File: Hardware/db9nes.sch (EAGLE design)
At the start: 3 parts

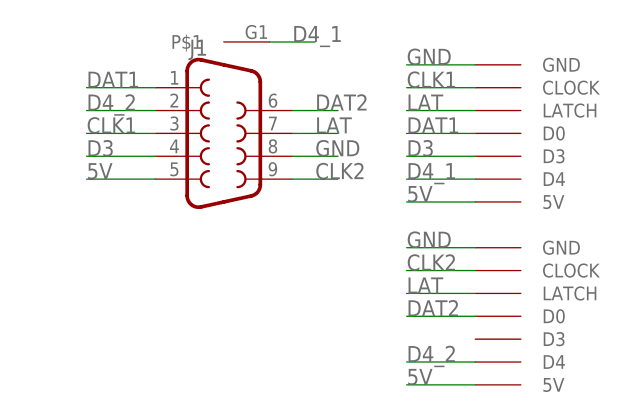
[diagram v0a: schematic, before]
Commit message: updated
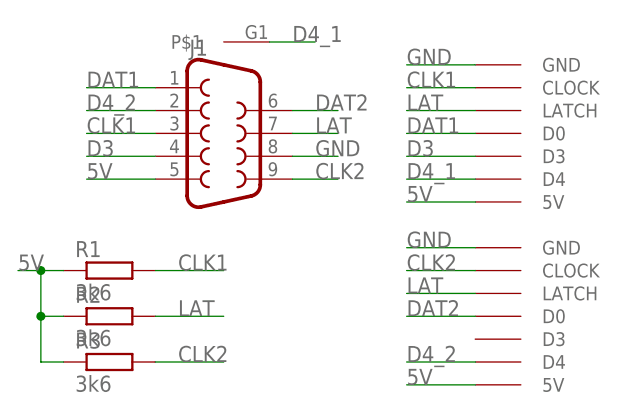
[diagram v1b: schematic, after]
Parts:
- added R1, R2, R3: 3k6, resistor:R-EU_R0603
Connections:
- net 5V: now also R1.1, R2.1, R3.1
- net CLK1: now also R1.2
- net CLK2: now also R3.2
- net LAT: now also R2.2
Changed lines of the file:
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@@
 <part name="U$2" library="gamepad-conn" deviceset="NESCONN" device="NO_TABS" value="NESCONNNO_TABS"/>
 <part name="U$1" library="gamepad-conn" deviceset="NESCONN" device="NO_TABS" value="NESCONNNO_TABS"/>
+<part name="R1" library="resistor" library_urn="urn:adsk.eagle:library:348" deviceset="R-EU_" device="R0603" package3d_urn="urn:adsk.eagle:package:26057/1" value="3k6"/>
+<part name="R2" library="resistor" library_urn="urn:adsk.eagle:library:348" deviceset="R-EU_" device="R0603" package3d_urn="urn:adsk.eagle:package:26057/1" value="3k6"/>
+<part name="R3" library="resistor" library_urn="urn:adsk.eagle:library:348" deviceset="R-EU_" device="R0603" package3d_urn="urn:adsk.eagle:package:26057/1" value="3k6"/>
 </parts>
 <sheets>
@@
 <instance part="U$2" gate="G$1" x="10.16" y="60.96"/>
 <instance part="U$1" gate="G$1" x="10.16" y="40.64"/>
+<instance part="R1" gate="G$1" x="-27.94" y="45.72"/>
+<instance part="R2" gate="G$1" x="-27.94" y="40.64"/>
+<instance part="R3" gate="G$1" x="-27.94" y="35.56"/>
 </instances>
 <busses>
@@
 <pinref part="U$1" gate="G$1" pin="5V"/>
 </segment>
+<segment>
+<pinref part="R1" gate="G$1" pin="1"/>
+<wire x1="-33.02" y1="45.72" x2="-35.56" y2="45.72" width="0.1524" layer="91"/>
+<label x="-38.1" y="45.72" size="1.778" layer="95"/>
+<wire x1="-35.56" y1="45.72" x2="-38.1" y2="45.72" width="0.1524" layer="91"/>
+<junction x="-35.56" y="45.72"/>
+<pinref part="R2" gate="G$1" pin="1"/>
+<wire x1="-35.56" y1="35.56" x2="-35.56" y2="40.64" width="0.1524" layer="91"/>
+<wire x1="-35.56" y1="40.64" x2="-35.56" y2="45.72" width="0.1524" layer="91"/>
+<wire x1="-33.02" y1="40.64" x2="-35.56" y2="40.64" width="0.1524" layer="91"/>
+<junction x="-35.56" y="40.64"/>
+<pinref part="R3" gate="G$1" pin="1"/>
+<wire x1="-33.02" y1="35.56" x2="-35.56" y2="35.56" width="0.1524" layer="91"/>
+</segment>
 </net>
 <net name="CLK1" class="0">
@@
 <label x="-30.48" y="60.96" size="1.778" layer="95"/>
 </segment>
+<segment>
+<pinref part="R1" gate="G$1" pin="2"/>
+<wire x1="-22.86" y1="45.72" x2="-15.24" y2="45.72" width="0.1524" layer="91"/>
+<label x="-20.32" y="45.72" size="1.778" layer="95"/>
+</segment>
 </net>
 <net name="DAT1" class="0">
@@
 <pinref part="U$1" gate="G$1" pin="LATCH"/>
 </segment>
+<segment>
+<pinref part="R2" gate="G$1" pin="2"/>
+<wire x1="-22.86" y1="40.64" x2="-15.24" y2="40.64" width="0.1524" layer="91"/>
+<label x="-20.32" y="40.64" size="1.778" layer="95"/>
+</segment>
 </net>
 <net name="DAT2" class="0">
@@
 <label x="5.08" y="45.72" size="1.778" layer="95"/>
 <pinref part="U$1" gate="G$1" pin="CLOCK"/>
+</segment>
+<segment>
+<pinref part="R3" gate="G$1" pin="2"/>
+<wire x1="-22.86" y1="35.56" x2="-15.24" y2="35.56" width="0.1524" layer="91"/>
+<label x="-20.32" y="35.56" size="1.778" layer="95"/>
 </segment>
 </net>
@@
 </schematic>
 </drawing>
+<compatibility>
+<note version="8.2" severity="warning">
+Since Version 8.2, EAGLE supports online libraries. The ids
+of those online libraries will not be understood (or retained)
+with this version.
+</note>
+<note version="8.3" severity="warning">
+Since Version 8.3, EAGLE supports URNs for individual library
+assets (packages, symbols, and devices). The URNs of those assets
+will not be understood (or retained) with this version.
+</note>
+<note version="8.3" severity="warning">
+Since Version 8.3, EAGLE supports the association of 3D packages
+with devices in libraries, schematics, and board files. Those 3D
+packages will not be understood (or retained) with this version.
+</note>
+</compatibility>
 </eagle>
